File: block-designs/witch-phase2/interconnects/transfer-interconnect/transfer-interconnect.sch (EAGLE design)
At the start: 60 parts, among them IC1 74LVC1G14DBV, IC10 74LVC1G14DBV, IC11 74LVC1G14DBV, IC12 74LVC1G14DBV, IC2 74LVC1G14DBV, IC3 74LVC1G14DBV, IC4 74LVC1G14DBV, IC5 74LVC1G14DBV, IC6 74LVC1G14DBV, IC7 74LVC1G14DBV, IC8 74LVC1G14DBV, IC9 74LVC1G14DBV

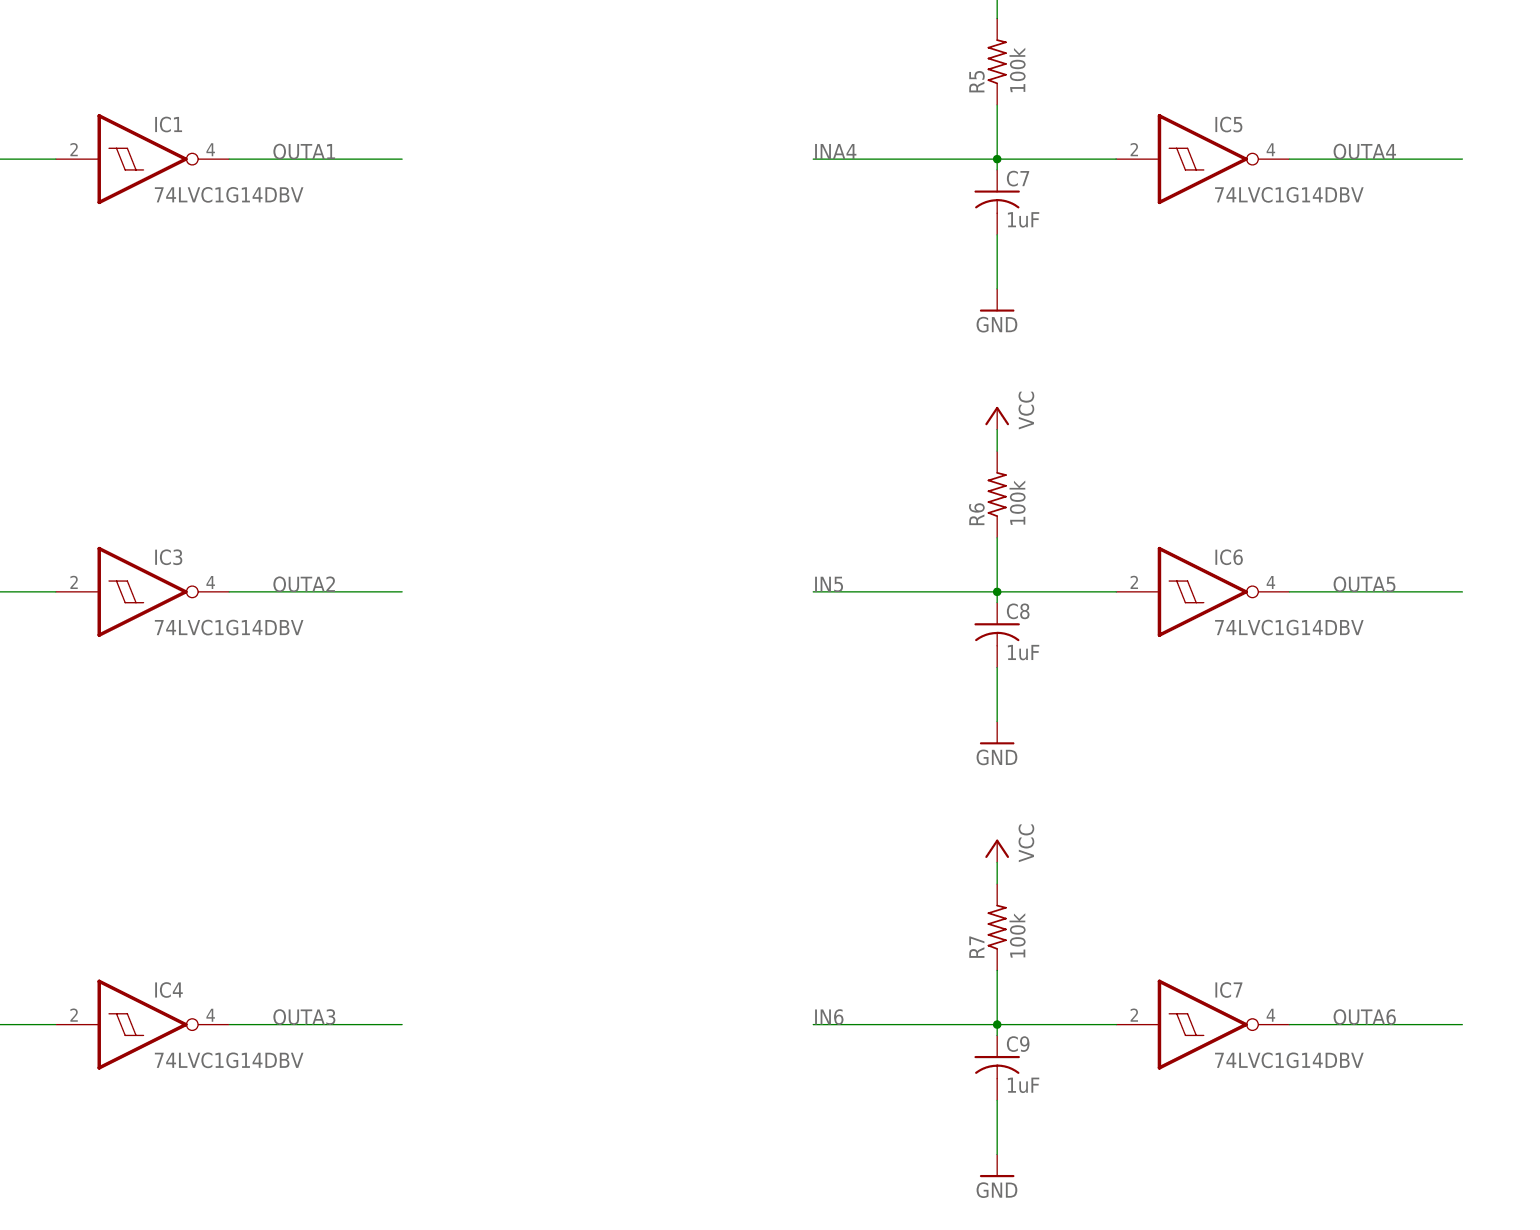
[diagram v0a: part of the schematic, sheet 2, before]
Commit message: minor cleanup
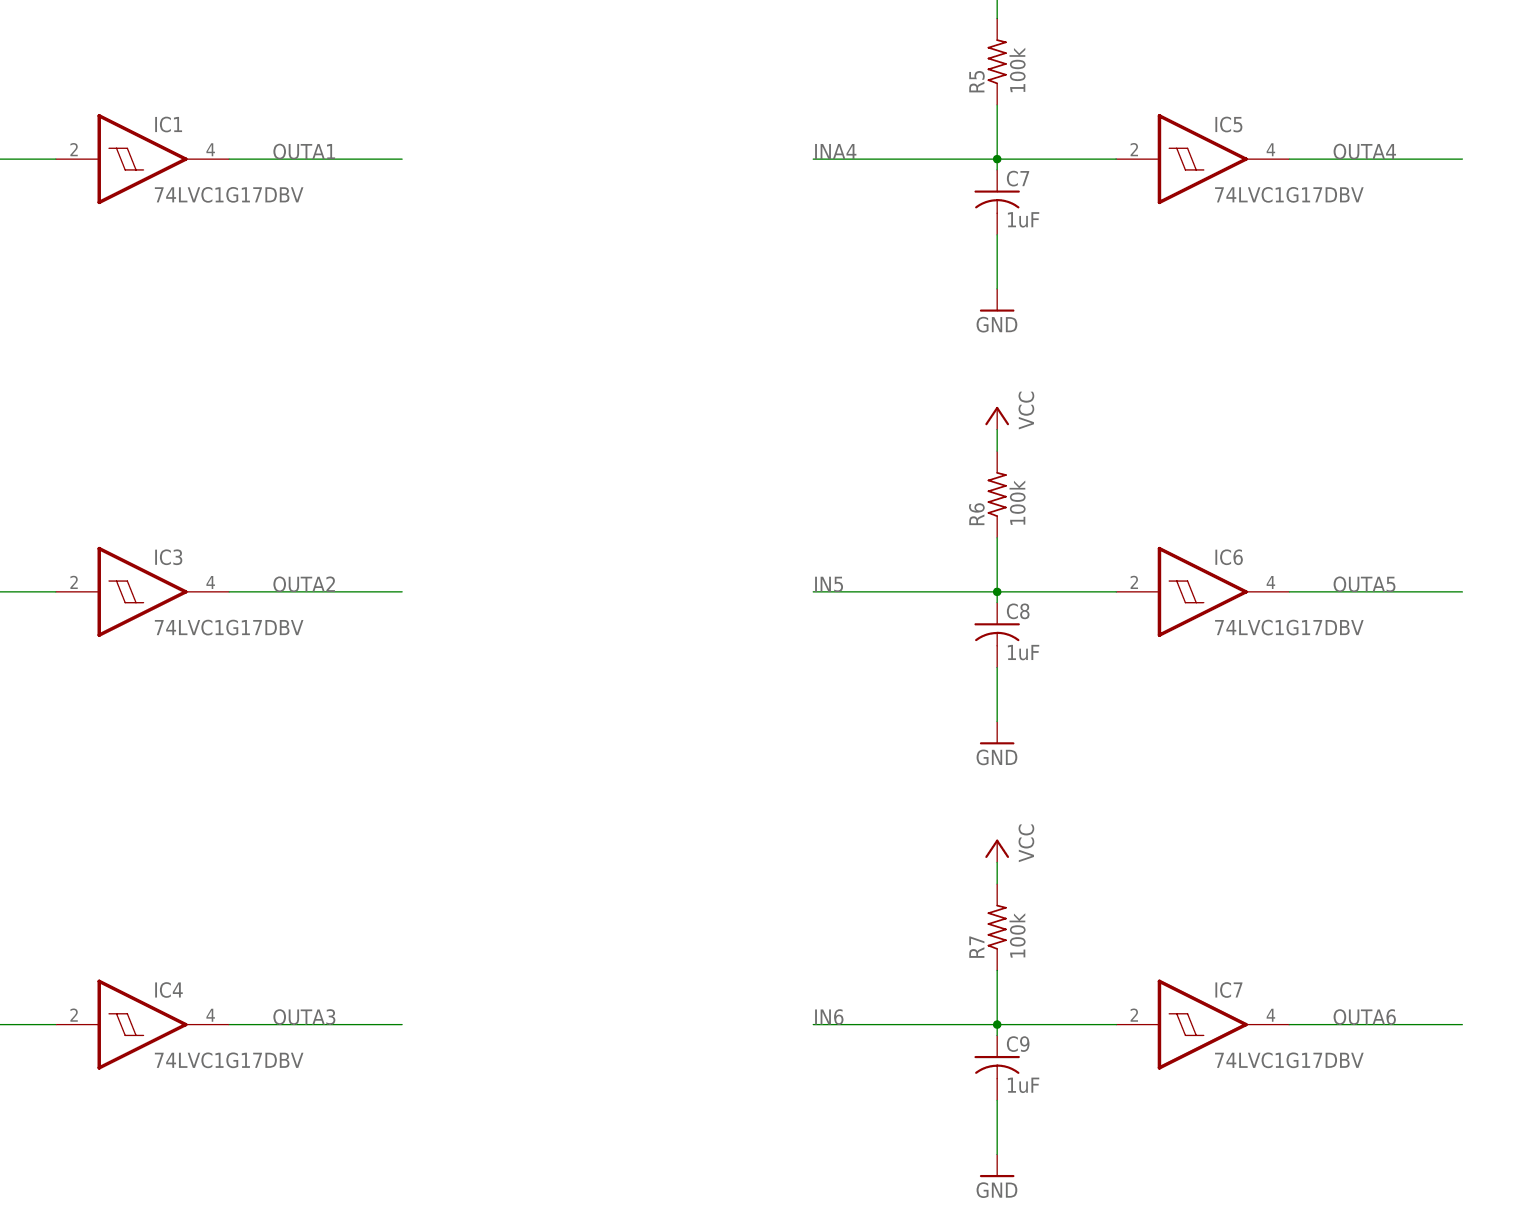
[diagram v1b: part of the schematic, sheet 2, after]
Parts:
- IC1, IC10, IC11, IC12, IC2, IC3, IC4, IC5, IC6, IC7, IC8, IC9: value 74LVC1G14DBV -> 74LVC1G17DBV; device 74xx-little-us:74LVC1G14DBV -> 74xx-little-us:74LVC1G17DBV
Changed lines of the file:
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@@
 <part name="P+7" library="supply1" deviceset="VCC" device=""/>
 <part name="R1" library="resistor" deviceset="R-US_" device="R0603" value="100k"/>
-<part name="IC1" library="74xx-little-us" deviceset="74*1G14" device="DBV" technology="LVC"/>
+<part name="IC1" library="74xx-little-us" deviceset="74*1G17" device="DBV" technology="LVC"/>
 <part name="FRAME2" library="frames" deviceset="TABL_L" device=""/>
 <part name="C5" library="resistor" deviceset="C-US" device="C0603K" value="1uF"/>
@@
 <part name="P+8" library="supply1" deviceset="VCC" device=""/>
 <part name="R3" library="resistor" deviceset="R-US_" device="R0603" value="100k"/>
-<part name="IC3" library="74xx-little-us" deviceset="74*1G14" device="DBV" technology="LVC"/>
+<part name="IC3" library="74xx-little-us" deviceset="74*1G17" device="DBV" technology="LVC"/>
 <part name="C6" library="resistor" deviceset="C-US" device="C0603K" value="1uF"/>
 <part name="GND9" library="supply1" deviceset="GND" device=""/>
 <part name="P+9" library="supply1" deviceset="VCC" device=""/>
 <part name="R4" library="resistor" deviceset="R-US_" device="R0603" value="100k"/>
-<part name="IC4" library="74xx-little-us" deviceset="74*1G14" device="DBV" technology="LVC"/>
+<part name="IC4" library="74xx-little-us" deviceset="74*1G17" device="DBV" technology="LVC"/>
 <part name="C7" library="resistor" deviceset="C-US" device="C0603K" value="1uF"/>
 <part name="GND10" library="supply1" deviceset="GND" device=""/>
 <part name="P+10" library="supply1" deviceset="VCC" device=""/>
 <part name="R5" library="resistor" deviceset="R-US_" device="R0603" value="100k"/>
-<part name="IC5" library="74xx-little-us" deviceset="74*1G14" device="DBV" technology="LVC"/>
+<part name="IC5" library="74xx-little-us" deviceset="74*1G17" device="DBV" technology="LVC"/>
 <part name="C8" library="resistor" deviceset="C-US" device="C0603K" value="1uF"/>
 <part name="GND11" library="supply1" deviceset="GND" device=""/>
 <part name="P+11" library="supply1" deviceset="VCC" device=""/>
 <part name="R6" library="resistor" deviceset="R-US_" device="R0603" value="100k"/>
-<part name="IC6" library="74xx-little-us" deviceset="74*1G14" device="DBV" technology="LVC"/>
+<part name="IC6" library="74xx-little-us" deviceset="74*1G17" device="DBV" technology="LVC"/>
 <part name="C9" library="resistor" deviceset="C-US" device="C0603K" value="1uF"/>
 <part name="GND12" library="supply1" deviceset="GND" device=""/>
 <part name="P+12" library="supply1" deviceset="VCC" device=""/>
 <part name="R7" library="resistor" deviceset="R-US_" device="R0603" value="100k"/>
-<part name="IC7" library="74xx-little-us" deviceset="74*1G14" device="DBV" technology="LVC"/>
+<part name="IC7" library="74xx-little-us" deviceset="74*1G17" device="DBV" technology="LVC"/>
 <part name="FRAME3" library="frames" deviceset="TABL_L" device=""/>
 <part name="C3" library="resistor" deviceset="C-US" device="C0603K" value="1uF"/>
@@
 <part name="P+6" library="supply1" deviceset="VCC" device=""/>
 <part name="R2" library="resistor" deviceset="R-US_" device="R0603" value="100k"/>
-<part name="IC2" library="74xx-little-us" deviceset="74*1G14" device="DBV" technology="LVC"/>
+<part name="IC2" library="74xx-little-us" deviceset="74*1G17" device="DBV" technology="LVC"/>
 <part name="C10" library="resistor" deviceset="C-US" device="C0603K" value="1uF"/>
 <part name="GND13" library="supply1" deviceset="GND" device=""/>
 <part name="P+13" library="supply1" deviceset="VCC" device=""/>
 <part name="R8" library="resistor" deviceset="R-US_" device="R0603" value="100k"/>
-<part name="IC8" library="74xx-little-us" deviceset="74*1G14" device="DBV" technology="LVC"/>
+<part name="IC8" library="74xx-little-us" deviceset="74*1G17" device="DBV" technology="LVC"/>
 <part name="C11" library="resistor" deviceset="C-US" device="C0603K" value="1uF"/>
 <part name="GND14" library="supply1" deviceset="GND" device=""/>
 <part name="P+14" library="supply1" deviceset="VCC" device=""/>
 <part name="R9" library="resistor" deviceset="R-US_" device="R0603" value="100k"/>
-<part name="IC9" library="74xx-little-us" deviceset="74*1G14" device="DBV" technology="LVC"/>
+<part name="IC9" library="74xx-little-us" deviceset="74*1G17" device="DBV" technology="LVC"/>
 <part name="C12" library="resistor" deviceset="C-US" device="C0603K" value="1uF"/>
 <part name="GND15" library="supply1" deviceset="GND" device=""/>
 <part name="P+15" library="supply1" deviceset="VCC" device=""/>
 <part name="R10" library="resistor" deviceset="R-US_" device="R0603" value="100k"/>
-<part name="IC10" library="74xx-little-us" deviceset="74*1G14" device="DBV" technology="LVC"/>
+<part name="IC10" library="74xx-little-us" deviceset="74*1G17" device="DBV" technology="LVC"/>
 <part name="C13" library="resistor" deviceset="C-US" device="C0603K" value="1uF"/>
 <part name="GND16" library="supply1" deviceset="GND" device=""/>
 <part name="P+16" library="supply1" deviceset="VCC" device=""/>
 <part name="R11" library="resistor" deviceset="R-US_" device="R0603" value="100k"/>
-<part name="IC11" library="74xx-little-us" deviceset="74*1G14" device="DBV" technology="LVC"/>
+<part name="IC11" library="74xx-little-us" deviceset="74*1G17" device="DBV" technology="LVC"/>
 <part name="C14" library="resistor" deviceset="C-US" device="C0603K" value="1uF"/>
 <part name="GND17" library="supply1" deviceset="GND" device=""/>
 <part name="P+17" library="supply1" deviceset="VCC" device=""/>
 <part name="R12" library="resistor" deviceset="R-US_" device="R0603" value="100k"/>
-<part name="IC12" library="74xx-little-us" deviceset="74*1G14" device="DBV" technology="LVC"/>
+<part name="IC12" library="74xx-little-us" deviceset="74*1G17" device="DBV" technology="LVC"/>
 <part name="C15" library="resistor" deviceset="C-US" device="C0603K" value="1uF"/>
 <part name="GND18" library="supply1" deviceset="GND" device=""/>
